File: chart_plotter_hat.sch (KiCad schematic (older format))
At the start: 46 parts, among them J1 JST PH, J2 JST PH, J3 40HAT, J4 JST PH, J5 JST PH, J6 JST PH, J7 JST PH, J8 Conn_02x03_Odd_Even, J9 JST PH, Q1 DMG2305UX, Q2 DMMT5401, U1 ATmega328P-AU, U2 CAT24C32, U3 MPM3610-adafruit, U4 LT1762, U5 G3VM-201FR

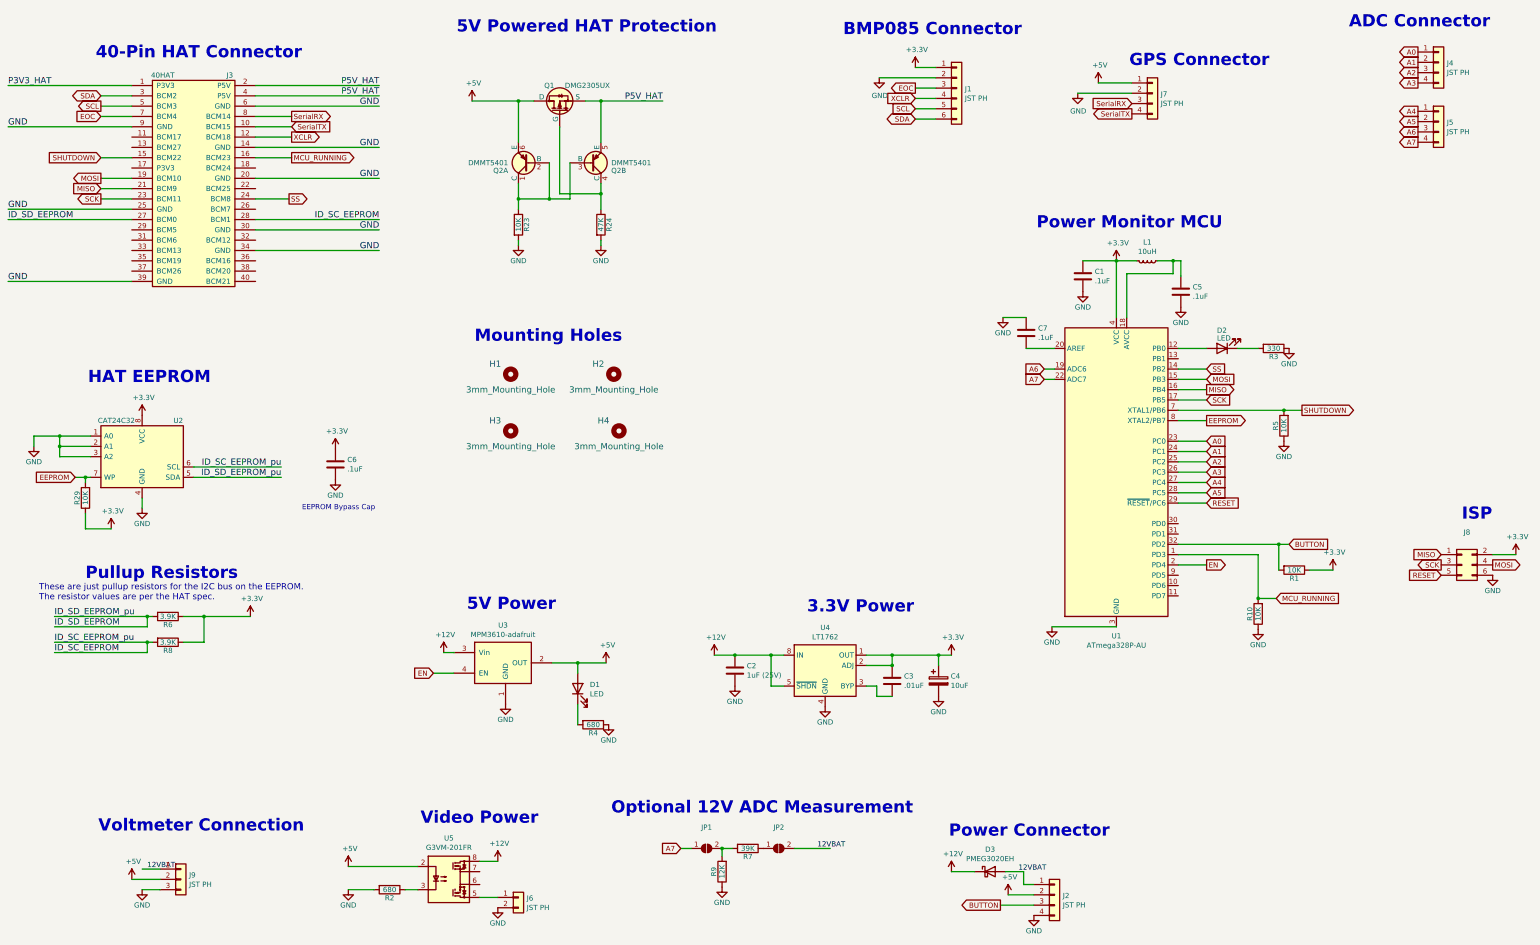
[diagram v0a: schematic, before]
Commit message: Added pdf of original release
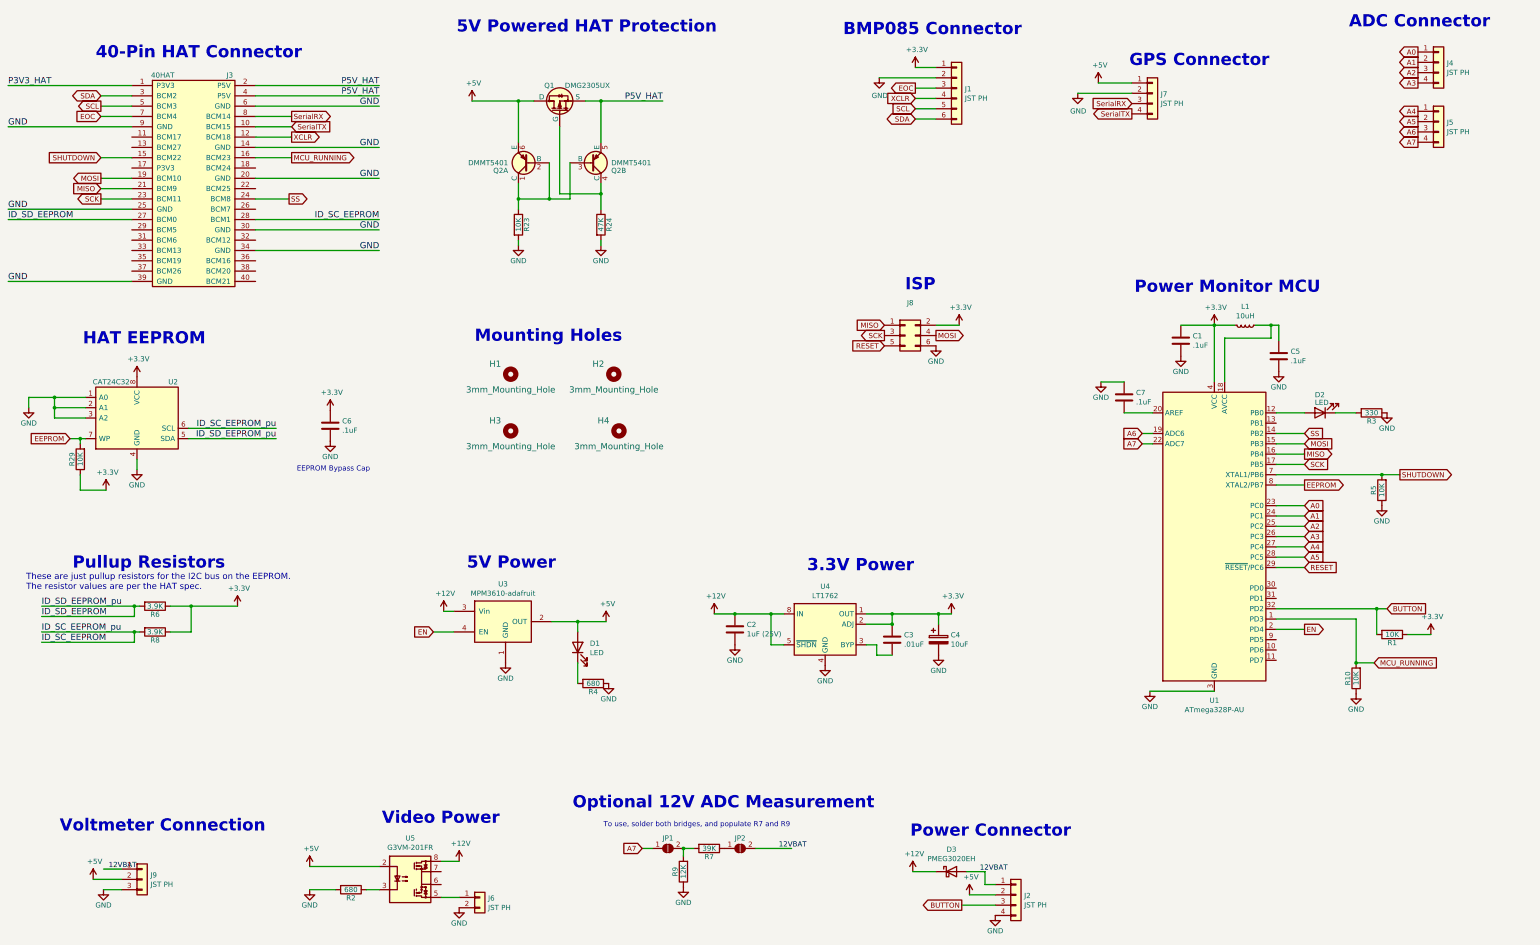
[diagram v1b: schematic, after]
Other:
- note added: "To use, solder both bridges, and populate R7 and R9"
- moved on the sheet: C1, C2, C3, C4, C5, C6, C7, D1, D2, D3, J2, J6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
